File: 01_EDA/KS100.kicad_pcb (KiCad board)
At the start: 2 copper layers, 80 x 80 mm, 55 parts, among them J1 Conn_01x02_Pin, J2 Conn_01x04, J3 DEM 128064E1 FGH, SW1 SW_Push, SW10 SW_Push, SW11 SW_Push, SW12 SW_Push, SW13 SW_Push, SW14 SW_Push, SW15 SW_Push, SW16 SW_Push, SW17 SW_Push, SW18 SW_Push, SW19 SW_Push, SW2 SW_Push, SW20 SW_Push, SW21 SW_Push, SW22 SW_Push, SW23 SW_Push, SW24 SW_Push, SW25 SW_Push, SW26 SW_Push, SW27 SW_Push, SW28 SW_Push, SW29 SW_Push, SW3 SW_Push, SW30 SW_Push, SW31 SW_Push, SW4 SW_Push, SW5 SW_Push, SW6 SW_Push, SW7 SW_Push, SW8 SW_Push, SW9 SW_Push, U1 STM32L071RZTx

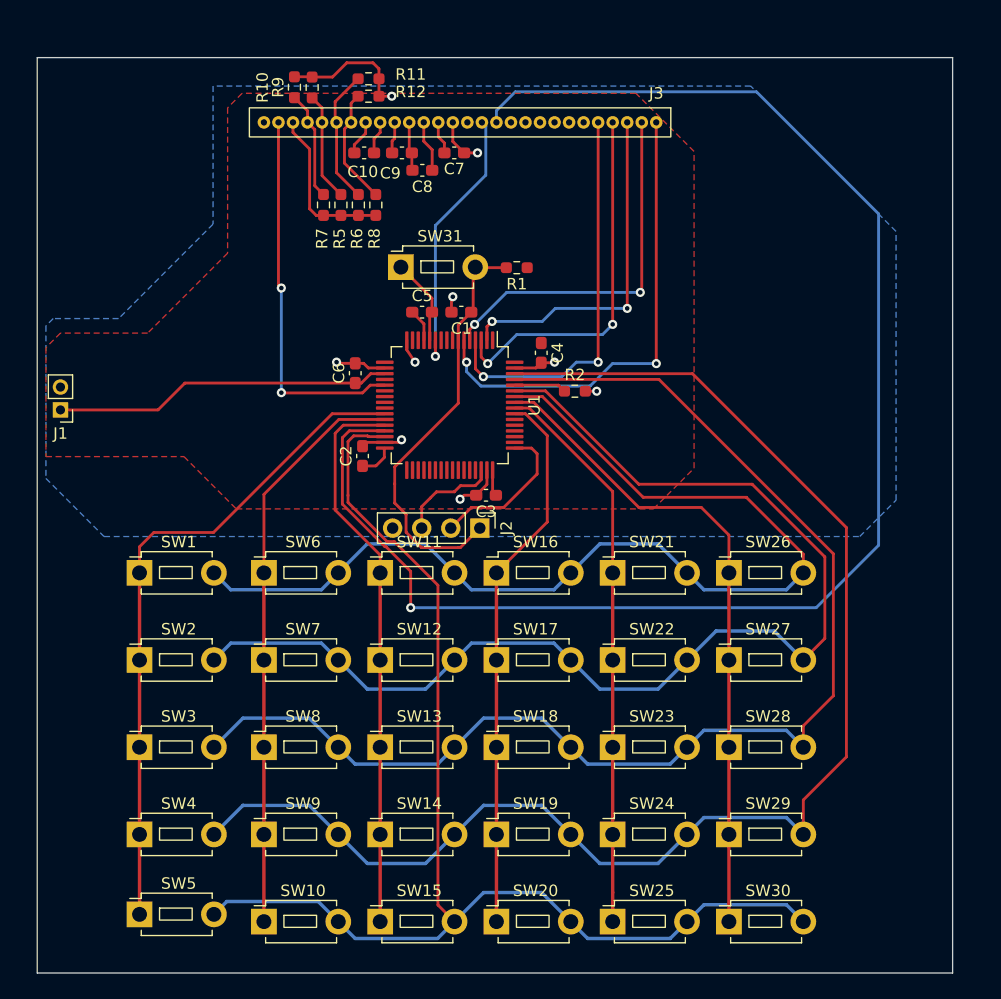
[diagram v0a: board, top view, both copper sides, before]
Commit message: Update.
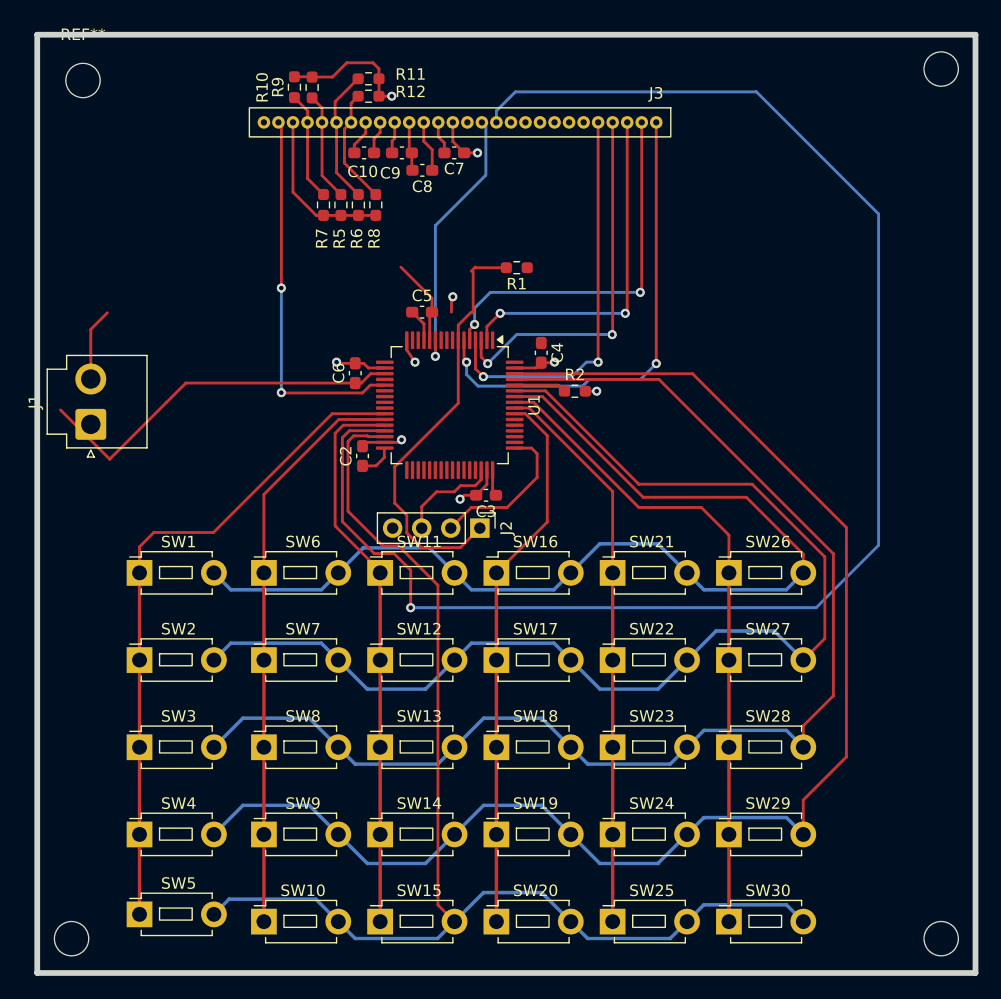
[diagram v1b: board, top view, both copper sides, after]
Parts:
- removed C1: C, Capacitor_SMD:C_0603_1608Metric_Pad1.08x0.95mm_HandSolder
- removed SW31: SW_Push, Button_Switch_THT:SW_PUSH_1P1T_6x3.5mm_H4.3_APEM_MJTP1243
- added ?: , , F.Cu at (190.0, 69.0)
- added ?: , , F.Cu at (190.0, 145.0)
- added ?: , , F.Cu at (114.0, 145.0)
- added REF**: MountingHole_3mm, MountingHole:MountingHole_3mm, F.Cu at (115.0, 70.0)
- J1: footprint Connector_PinHeader_2.00mm:PinHeader_1x02_P2.00mm_Vertical -> Connector_JST:JST_VH_B2P-VH-B_1x02_P3.96mm_Vertical
- moved J1 2.93 mm to (115.7, 100.0), turned to 90 degrees
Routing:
- net GND: track 41.8 -> 48.2 mm
- net +BATT: track 37.9 -> 41.5 mm
- net /Calculator/SCL: track 133.0 -> 133.9 mm
- net /Calculator/LCD_RST: track 32.1 -> 32.9 mm
- net /Calculator/Y5: track 108.1 -> 108.7 mm
- net /Calculator/WR: track 32.3 -> 32.8 mm
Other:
- board size 80 x 80 mm -> 82 x 82 mm
